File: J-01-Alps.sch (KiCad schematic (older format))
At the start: 17 parts, among them SW1 SW_Push, U1 ATmega32U4-AU, U4 PRTR5V0U2X, Y1 16MHz

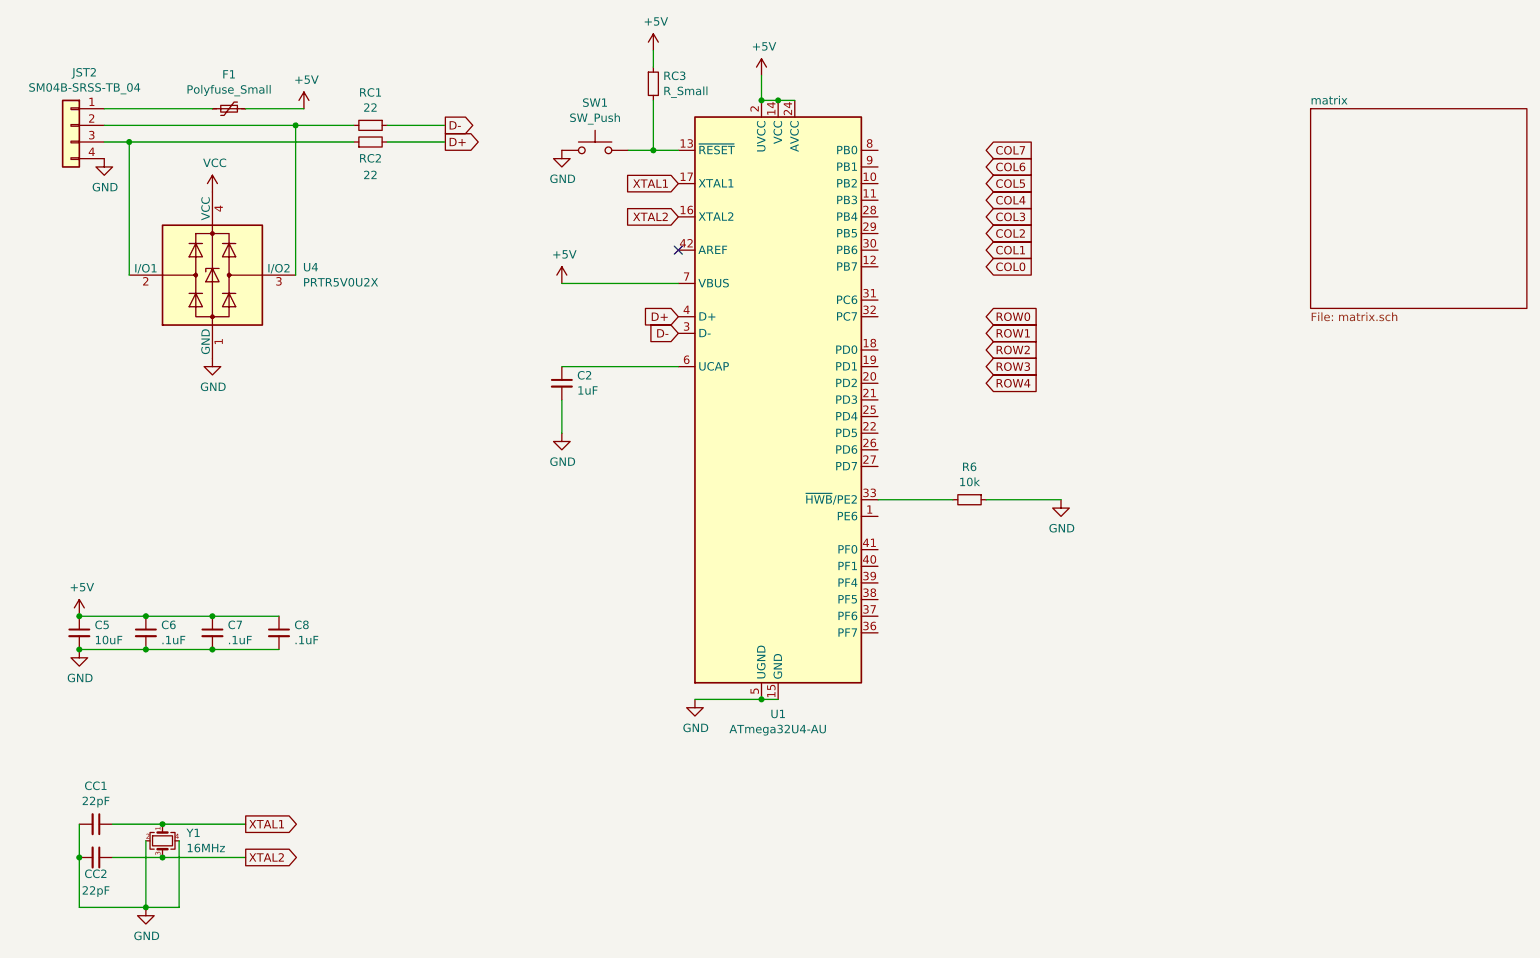
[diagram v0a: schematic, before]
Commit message: Bugfixes
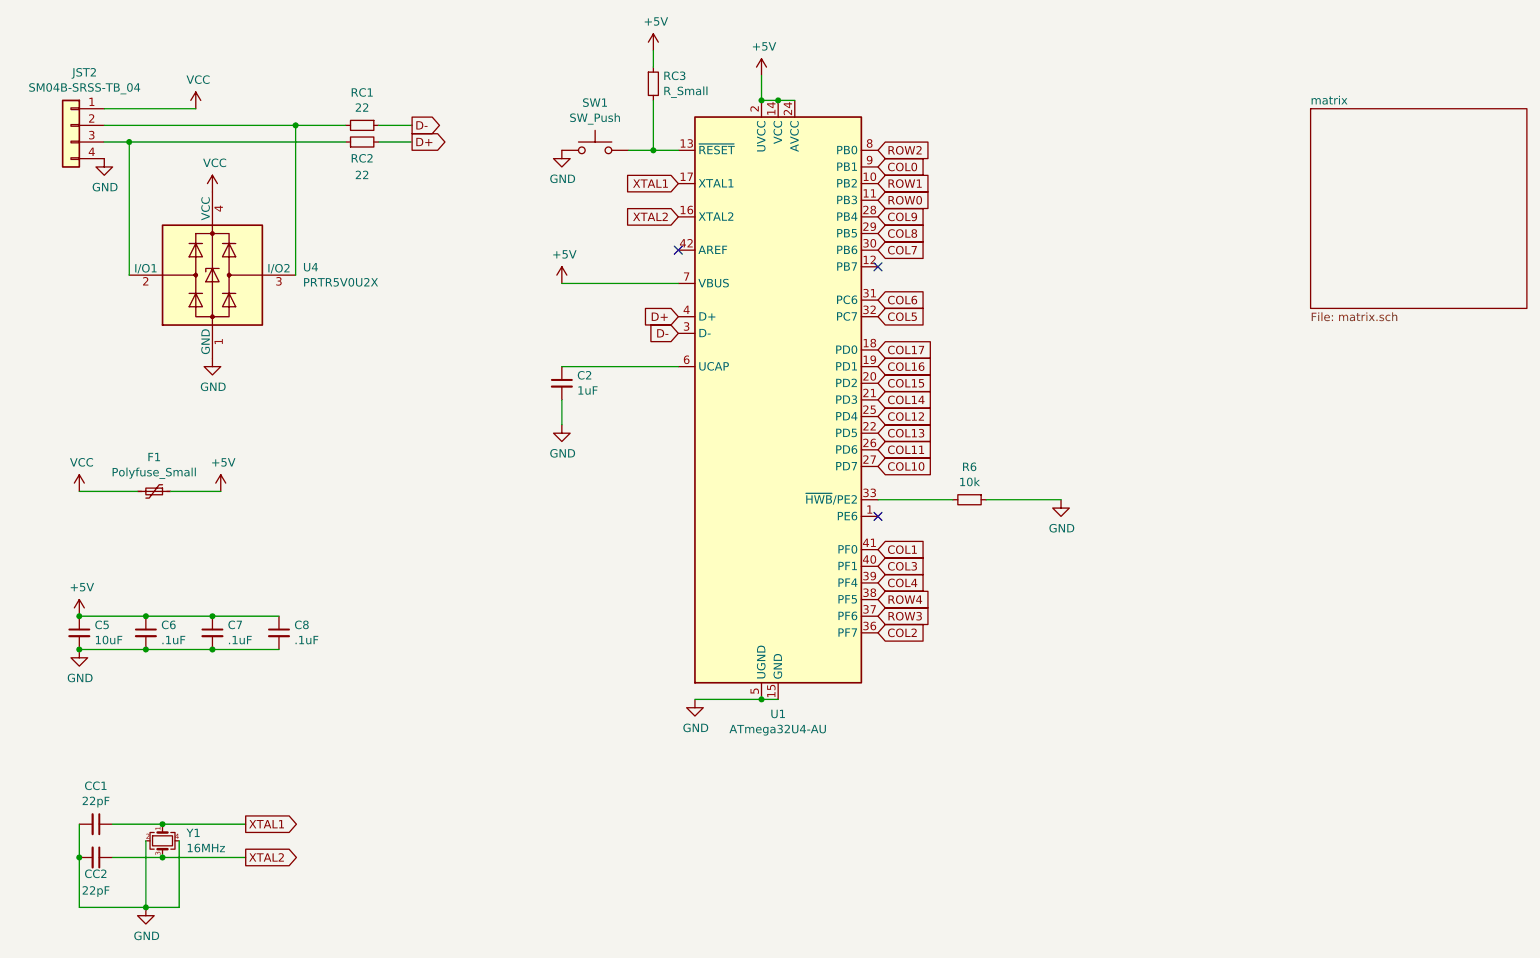
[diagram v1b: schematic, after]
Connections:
- net COL0: now also U1.9 (PB1)
- net COL1: now also U1.41 (PF0)
- net COL2: now also U1.36 (PF7)
- net COL3: now also U1.40 (PF1)
- net COL4: now also U1.39 (PF4)
- net COL5: now also U1.32 (PC7)
- net COL6: now also U1.31 (PC6)
- net COL7: now also U1.30 (PB6)
- net ROW0: now also U1.11 (PB3)
- net ROW1: now also U1.10 (PB2)
- net ROW2: now also U1.8 (PB0)
- net ROW3: now also U1.37 (PF6)
- net ROW4: now also U1.38 (PF5)
- net VCC: now also F1.2, JST2.1 (Pin_1)
- net COL17: now reaches U1.18 (PD0)
- net COL16: now reaches U1.19 (PD1)
- net COL15: now reaches U1.20 (PD2)
- net COL14: now reaches U1.21 (PD3)
- net COL13: now reaches U1.22 (PD5)
- net COL12: now reaches U1.25 (PD4)
- net COL11: now reaches U1.26 (PD6)
- net COL10: now reaches U1.27 (PD7)
- net COL9: now reaches U1.28 (PB4)
- net COL8: now reaches U1.29 (PB5)
- no-connect marks 1 -> 3
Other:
- moved on the sheet: F1, RC1, RC2
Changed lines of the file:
@@
 L power:GND #PWR0104
 U 1 1 61BC5372
-P 4200 3350
-F 0 "#PWR0104" H 4200 3100 50  0001 C CNN
-F 1 "GND" H 4205 3177 50  0000 C CNN
-F 2 "" H 4200 3350 50  0001 C CNN
-F 3 "" H 4200 3350 50  0001 C CNN
-	1    4200 3350
-	1    0    0    -1
-$EndComp
-Wire Wire Line
-	4200 3350 4200 3150
+P 4200 3300
+F 0 "#PWR0104" H 4200 3050 50  0001 C CNN
+F 1 "GND" H 4205 3127 50  0000 C CNN
+F 2 "" H 4200 3300 50  0001 C CNN
+F 3 "" H 4200 3300 50  0001 C CNN
+	1    4200 3300
+	1    0    0    -1
+$EndComp
 $Comp
 L Connector_Generic:Conn_01x04 JST2
@@
 L Device:Polyfuse_Small F1
 U 1 1 61BC3615
-P 2200 1400
-F 0 "F1" V 1995 1400 50  0000 C CNN
-F 1 "Polyfuse_Small" V 2086 1400 50  0000 C CNN
-F 2 "Fuse:Fuse_1206_3216Metric_Pad1.42x1.75mm_HandSolder" H 2250 1200 50  0001 L CNN
-F 3 "~" H 2200 1400 50  0001 C CNN
-	1    2200 1400
+P 1750 3700
+F 0 "F1" V 1545 3700 50  0000 C CNN
+F 1 "Polyfuse_Small" V 1636 3700 50  0000 C CNN
+F 2 "Fuse:Fuse_1206_3216Metric_Pad1.42x1.75mm_HandSolder" H 1800 3500 50  0001 L CNN
+F 3 "~" H 1750 3700 50  0001 C CNN
+	1    1750 3700
 	0    1    1    0
 $EndComp
@@
 L Device:R_Small RC1
 U 1 1 61BC52CD
-P 3050 1500
-F 0 "RC1" V 2854 1500 50  0000 C CNN
-F 1 "22" V 2945 1500 50  0000 C CNN
-F 2 "Resistor_SMD:R_0603_1608Metric_Pad0.98x0.95mm_HandSolder" H 3050 1500 50  0001 C CNN
-F 3 "~" H 3050 1500 50  0001 C CNN
-	1    3050 1500
+P 3000 1500
+F 0 "RC1" V 2804 1500 50  0000 C CNN
+F 1 "22" V 2895 1500 50  0000 C CNN
+F 2 "Resistor_SMD:R_0603_1608Metric_Pad0.98x0.95mm_HandSolder" H 3000 1500 50  0001 C CNN
+F 3 "~" H 3000 1500 50  0001 C CNN
+	1    3000 1500
 	0    1    1    0
 $EndComp
@@
 L Device:R_Small RC2
 U 1 1 61BC5632
-P 3050 1600
-F 0 "RC2" V 2950 1600 50  0000 C CNN
-F 1 "22" V 2850 1600 50  0000 C CNN
-F 2 "Resistor_SMD:R_0603_1608Metric_Pad0.98x0.95mm_HandSolder" H 3050 1600 50  0001 C CNN
-F 3 "~" H 3050 1600 50  0001 C CNN
-	1    3050 1600
+P 3000 1600
+F 0 "RC2" V 2900 1600 50  0000 C CNN
+F 1 "22" V 2800 1600 50  0000 C CNN
+F 2 "Resistor_SMD:R_0603_1608Metric_Pad0.98x0.95mm_HandSolder" H 3000 1600 50  0001 C CNN
+F 3 "~" H 3000 1600 50  0001 C CNN
+	1    3000 1600
 	0    -1   -1   0
 $EndComp
-Text GLabel 3500 1500 2    50   Output ~ 0
+Text GLabel 3300 1500 2    50   Output ~ 0
 D-
-Text GLabel 3500 1600 2    50   Output ~ 0
+Text GLabel 3300 1600 2    50   Output ~ 0
 D+
 Wire Wire Line
-	3150 1500 3500 1500
-Wire Wire Line
-	3150 1600 3500 1600
+	3100 1500 3300 1500
+Wire Wire Line
+	3100 1600 3300 1600
 Text GLabel 4900 2650 0    50   Input ~ 0
 D+
@@
 L power:+5V #PWR0111
 U 1 1 61BE4541
-P 2650 1400
-F 0 "#PWR0111" H 2650 1250 50  0001 C CNN
-F 1 "+5V" H 2665 1573 50  0000 C CNN
-F 2 "" H 2650 1400 50  0001 C CNN
-F 3 "" H 2650 1400 50  0001 C CNN
-	1    2650 1400
-	1    0    0    -1
-$EndComp
-Wire Wire Line
-	2300 1400 2650 1400
+P 2150 3700
+F 0 "#PWR0111" H 2150 3550 50  0001 C CNN
+F 1 "+5V" H 2165 3873 50  0000 C CNN
+F 2 "" H 2150 3700 50  0001 C CNN
+F 3 "" H 2150 3700 50  0001 C CNN
+	1    2150 3700
+	1    0    0    -1
+$EndComp
+Wire Wire Line
+	1850 3700 2150 3700
 Wire Wire Line
 	1450 1500 2600 1500
@@
 Connection ~ 1600 1600
 Wire Wire Line
-	1600 1600 2950 1600
+	1600 1600 2900 1600
 Wire Wire Line
 	2600 2400 2600 1500
 Connection ~ 2600 1500
 Wire Wire Line
-	2600 1500 2950 1500
-$Comp
-L power:VCC #PWR0114
-U 1 1 61BEE6C5
-P 2100 1900
-F 0 "#PWR0114" H 2100 1750 50  0001 C CNN
-F 1 "VCC" H 2115 2073 50  0000 C CNN
-F 2 "" H 2100 1900 50  0001 C CNN
-F 3 "" H 2100 1900 50  0001 C CNN
-	1    2100 1900
-	1    0    0    -1
-$EndComp
+	2600 1500 2900 1500
 $Sheet
 S 8700 1400 1300 1200
@@
 F1 "matrix.sch" 50
 $EndSheet
-Text GLabel 6750 2650 2    50   Input ~ 0
+Text GLabel 6100 1950 2    50   Input ~ 0
 ROW0
-Text GLabel 6750 2750 2    50   Input ~ 0
+Text GLabel 6100 1850 2    50   Input ~ 0
 ROW1
-Text GLabel 6750 2850 2    50   Input ~ 0
+Text GLabel 6100 1650 2    50   Input ~ 0
 ROW2
-Text GLabel 6750 2950 2    50   Input ~ 0
+Text GLabel 6100 4450 2    50   Input ~ 0
 ROW3
-Text GLabel 6750 3050 2    50   Input ~ 0
+Text GLabel 6100 4350 2    50   Input ~ 0
 ROW4
-Text GLabel 6750 2350 2    50   Input ~ 0
+Text GLabel 6100 1750 2    50   Input ~ 0
 COL0
-Text GLabel 6750 2250 2    50   Input ~ 0
+Text GLabel 6100 4050 2    50   Input ~ 0
 COL1
-Text GLabel 6750 2150 2    50   Input ~ 0
+Text GLabel 6100 4550 2    50   Input ~ 0
 COL2
-Text GLabel 6750 2050 2    50   Input ~ 0
+Text GLabel 6100 4150 2    50   Input ~ 0
 COL3
-Text GLabel 6750 1950 2    50   Input ~ 0
+Text GLabel 6100 4250 2    50   Input ~ 0
 COL4
-Text GLabel 6750 1850 2    50   Input ~ 0
+Text GLabel 6100 2650 2    50   Input ~ 0
 COL5
-Text GLabel 6750 1750 2    50   Input ~ 0
+Text GLabel 6100 2550 2    50   Input ~ 0
 COL6
-Text GLabel 6750 1650 2    50   Input ~ 0
+Text GLabel 6100 2250 2    50   Input ~ 0
 COL7
-Wire Wire Line
-	1450 1400 2100 1400
+Text GLabel 6100 2150 2    50   Input ~ 0
+COL8
+Text GLabel 6100 3450 2    50   Input ~ 0
+COL11
+Text GLabel 6100 3350 2    50   Input ~ 0
+COL13
+Text GLabel 6100 3250 2    50   Input ~ 0
+COL12
+Text GLabel 6100 2050 2    50   Input ~ 0
+COL9
+Text GLabel 6100 3550 2    50   Input ~ 0
+COL10
+Text GLabel 6100 3150 2    50   Input ~ 0
+COL14
+Text GLabel 6100 3050 2    50   Input ~ 0
+COL15
+Text GLabel 6100 2950 2    50   Input ~ 0
+COL16
+Text GLabel 6100 2850 2    50   Input ~ 0
+COL17
+NoConn ~ 6100 3850
+NoConn ~ 6100 2350
+$Comp
+L power:VCC #PWR0114
+U 1 1 61F1803F
+P 1300 3700
+F 0 "#PWR0114" H 1300 3550 50  0001 C CNN
+F 1 "VCC" H 1315 3873 50  0000 C CNN
+F 2 "" H 1300 3700 50  0001 C CNN
+F 3 "" H 1300 3700 50  0001 C CNN
+	1    1300 3700
+	1    0    0    -1
+$EndComp
+Wire Wire Line
+	1300 3700 1650 3700
+$Comp
+L power:VCC #PWR0115
+U 1 1 61F1B227
+P 2000 1400
+F 0 "#PWR0115" H 2000 1250 50  0001 C CNN
+F 1 "VCC" H 2015 1573 50  0000 C CNN
+F 2 "" H 2000 1400 50  0001 C CNN
+F 3 "" H 2000 1400 50  0001 C CNN
+	1    2000 1400
+	1    0    0    -1
+$EndComp
+Wire Wire Line
+	1450 1400 2000 1400
+$Comp
+L power:VCC #PWR0116
+U 1 1 61F1C94A
+P 2100 1900
+F 0 "#PWR0116" H 2100 1750 50  0001 C CNN
+F 1 "VCC" H 2115 2073 50  0000 C CNN
+F 2 "" H 2100 1900 50  0001 C CNN
+F 3 "" H 2100 1900 50  0001 C CNN
+	1    2100 1900
+	1    0    0    -1
+$EndComp
+Wire Wire Line
+	4200 3300 4200 3150
 $EndSCHEMATC
